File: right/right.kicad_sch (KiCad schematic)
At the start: 0 parts

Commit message: done right side
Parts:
- added C1: 4.7uF, Capacitor_SMD:C_0805_2012Metric_Pad1.18x1.45mm_HandSolder, symbol Device:C
- added C2, C4, C5: 0.1uF, Capacitor_SMD:C_0805_2012Metric_Pad1.18x1.45mm_HandSolder, symbol Device:C
- added C3, C6, C7: 1uF, Capacitor_SMD:C_0805_2012Metric_Pad1.18x1.45mm_HandSolder, symbol Device:C
- added D18: SS14, Diode_SMD:D_SMA, symbol Diode:SS14
- added F2: 1A, Fuse:Fuse_1206_3216Metric, symbol Device:Polyfuse
- added J2: USB_C_Receptacle_OUT, Connector_USB:USB_C_Receptacle_HRO_TYPE-C-31-M-12, symbol Connector:USB_C_Receptacle_USB2.0_16P
- added R1: 10k, Resistor_SMD:R_0805_2012Metric_Pad1.20x1.40mm_HandSolder, symbol Device:R
- added SW1: SW_Push, Button_Switch_SMD:SW_SPST_TS-1088-xR020, symbol Switch:SW_Push
- added SW2: SW_SPDT, Button_Switch_SMD:SW_SPDT_PCM12, symbol Switch:SW_SPDT
- added U1: STM32G0B1CBTx, Package_QFP:LQFP-48_7x7mm_P0.5mm, symbol MCU_ST_STM32G0:STM32G0B1CBTx
- added U2: SRV05-4, Package_TO_SOT_SMD:SOT-23-6, symbol Power_Protection:SRV05-4
- added U3: XC6206P332MR, Package_TO_SOT_SMD:SOT-23-3, symbol Regulator_Linear:XC6206PxxxMR
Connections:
- new net: R1.2, SW2.2 (B)
- new net: D18.1 (K), F2.1
- new net +3.3V: C1.1, C2.1, C3.1, C4.1, C7.1, SW2.3 (C), U1.4 (VBAT), U1.5 (VREF+), U1.6 (VDD), U2.5 (VP), U3.2 (VO)
- new net +5V: C6.1, F2.2, U3.3 (VI)
- new net BOOT0: R1.1, U1.36 (PA14)
- new net COL0: U1.37 (PA15)
- new net COL1: U1.38 (PD0)
- new net COL2: U1.39 (PD1)
- new net COL3: U1.40 (PD2)
- new net COL4: U1.41 (PD3)
- new net D+: U1.34 (PA10/PA12)
- new net D-: U1.33 (PA9/PA11)
- new net GND: C1.2, C2.2, C3.2, C4.2, C5.2, C6.2, C7.2, J2.A1 (GND), J2.A12 (GND), J2.B1 (GND), J2.B12 (GND), J2.SH (SHIELD), SW1.2, SW2.1 (A), U1.7 (VSS), U2.2 (VN), U3.1 (GND)
- new net ROW0: U1.47 (PB8)
- new net ROW1: U1.46 (PB7)
- new net ROW2: U1.45 (PB6)
- new net ROW3: U1.25 (PB13)
- new net RX: J2.A8 (SBU1), U1.27 (PB15), U2.1 (IO1)
- new net TX: J2.B8 (SBU2), U1.26 (PB14), U2.6 (IO4)
- new net VBUS: D18.2 (A), J2.A4 (VBUS), J2.A9 (VBUS), J2.B4 (VBUS), J2.B9 (VBUS)
- new net nRST: C5.1, SW1.1, U1.10 (PF2)
- no-connect marks 0 -> 6
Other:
- added sheet Switch Matrix (matrix.kicad_sch)

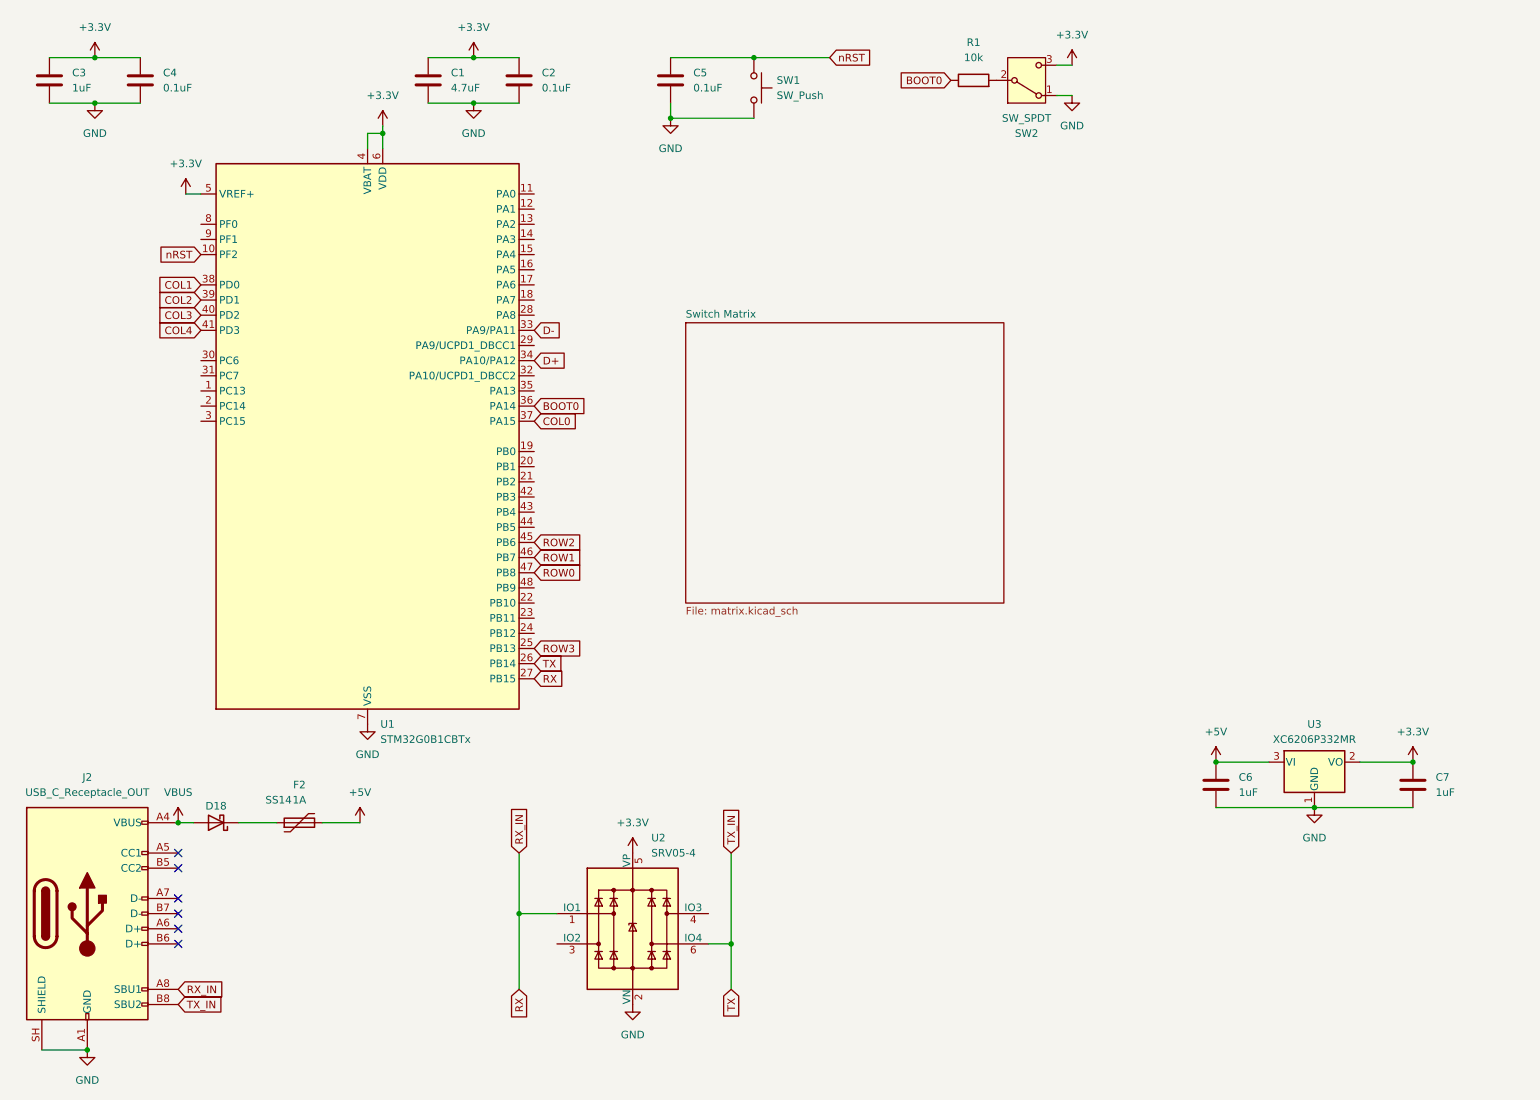
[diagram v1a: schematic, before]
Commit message: fixed schematics
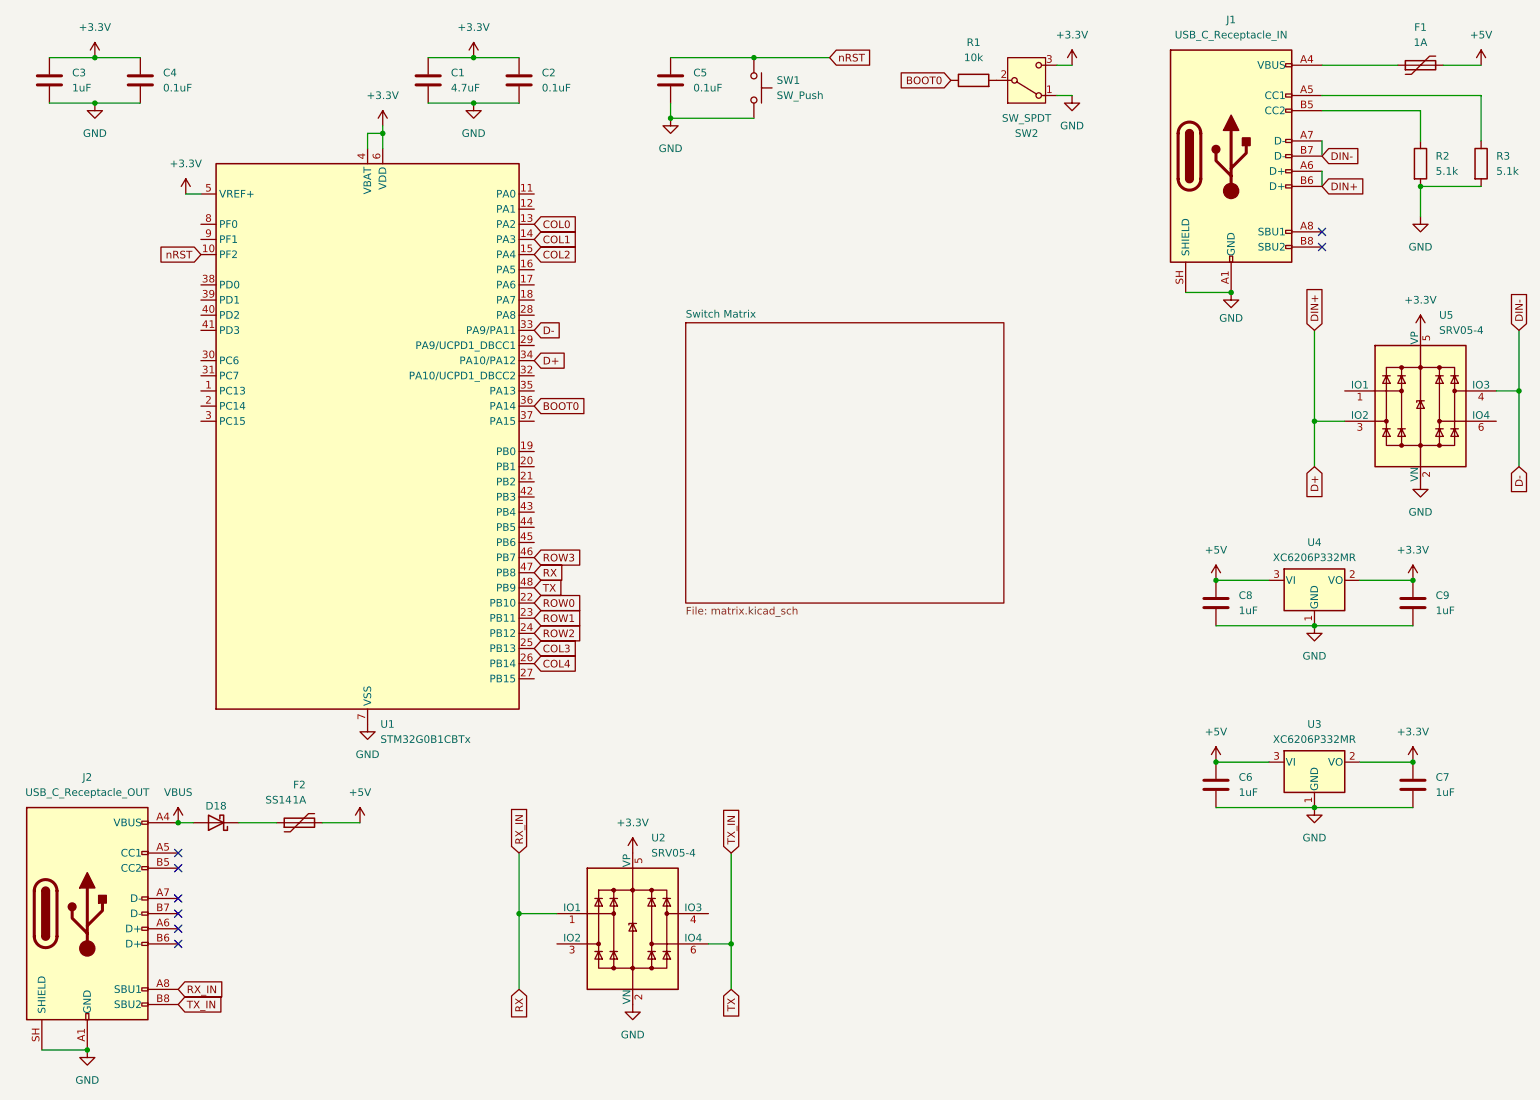
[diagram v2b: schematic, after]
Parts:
- added C8, C9: 1uF, Capacitor_SMD:C_0805_2012Metric_Pad1.18x1.45mm_HandSolder, symbol Device:C
- added F1: 1A, Fuse:Fuse_1206_3216Metric, symbol Device:Polyfuse
- added J1: USB_C_Receptacle_IN, Connector_USB:USB_C_Receptacle_HRO_TYPE-C-31-M-12, symbol Connector:USB_C_Receptacle_USB2.0_16P
- added R2, R3: 5.1k, Resistor_SMD:R_0805_2012Metric_Pad1.20x1.40mm_HandSolder, symbol Device:R
- added U4: XC6206P332MR, Package_TO_SOT_SMD:SOT-23-3, symbol Regulator_Linear:XC6206PxxxMR
- added U5: SRV05-4, Package_TO_SOT_SMD:SOT-23-6, symbol Power_Protection:SRV05-4
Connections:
- net +3.3V: now also C9.1, U4.2 (VO), U5.5 (VP)
- net +5V: now also C8.1, F1.2, U4.3 (VI)
- net COL0: now also U1.13 (PA2); no longer U1.37 (PA15)
- net COL1: now also U1.14 (PA3); no longer U1.38 (PD0)
- net COL2: now also U1.15 (PA4); no longer U1.39 (PD1)
- net COL3: now also U1.25 (PB13); no longer U1.40 (PD2)
- net COL4: now also U1.26 (PB14); no longer U1.41 (PD3)
- net D+: now also J1.A6 (D+), J1.B6 (D+), U5.3 (IO2)
- net D-: now also J1.A7 (D-), J1.B7 (D-), U5.4 (IO3)
- net GND: now also C8.2, C9.2, J1.A1 (GND), J1.A12 (GND), J1.B1 (GND), J1.B12 (GND), J1.SH (SHIELD), R2.2, R3.2, U4.1 (GND), U5.2 (VN)
- net ROW0: now also U1.22 (PB10); no longer U1.47 (PB8)
- net ROW1: now also U1.23 (PB11); no longer U1.46 (PB7)
- net ROW2: now also U1.24 (PB12); no longer U1.45 (PB6)
- net ROW3: now also U1.46 (PB7); no longer U1.25 (PB13)
- net RX: now also U1.47 (PB8); no longer U1.27 (PB15)
- net TX: now also U1.48 (PB9); no longer U1.26 (PB14)
- new net: J1.A5 (CC1), R3.1
- new net: F1.1, J1.A4 (VBUS), J1.A9 (VBUS), J1.B4 (VBUS), J1.B9 (VBUS)
- new net: J1.B5 (CC2), R2.1
- no-connect marks 6 -> 8
